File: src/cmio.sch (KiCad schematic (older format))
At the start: 28 parts, among them J1 CONN_01X02_MALE, J2 CONN_02X20, J3 USB_OTG, J4 CM3Lite, J5 CONN_COAXIAL, J6 CONN_02X20, J7 Micro_SD_Card_TFP09_2_12B, J8 CONN_01X06, SW1 SW_Push, U1 ISL91107IR, U2 LD3985M18R, U3 LD3985M28R

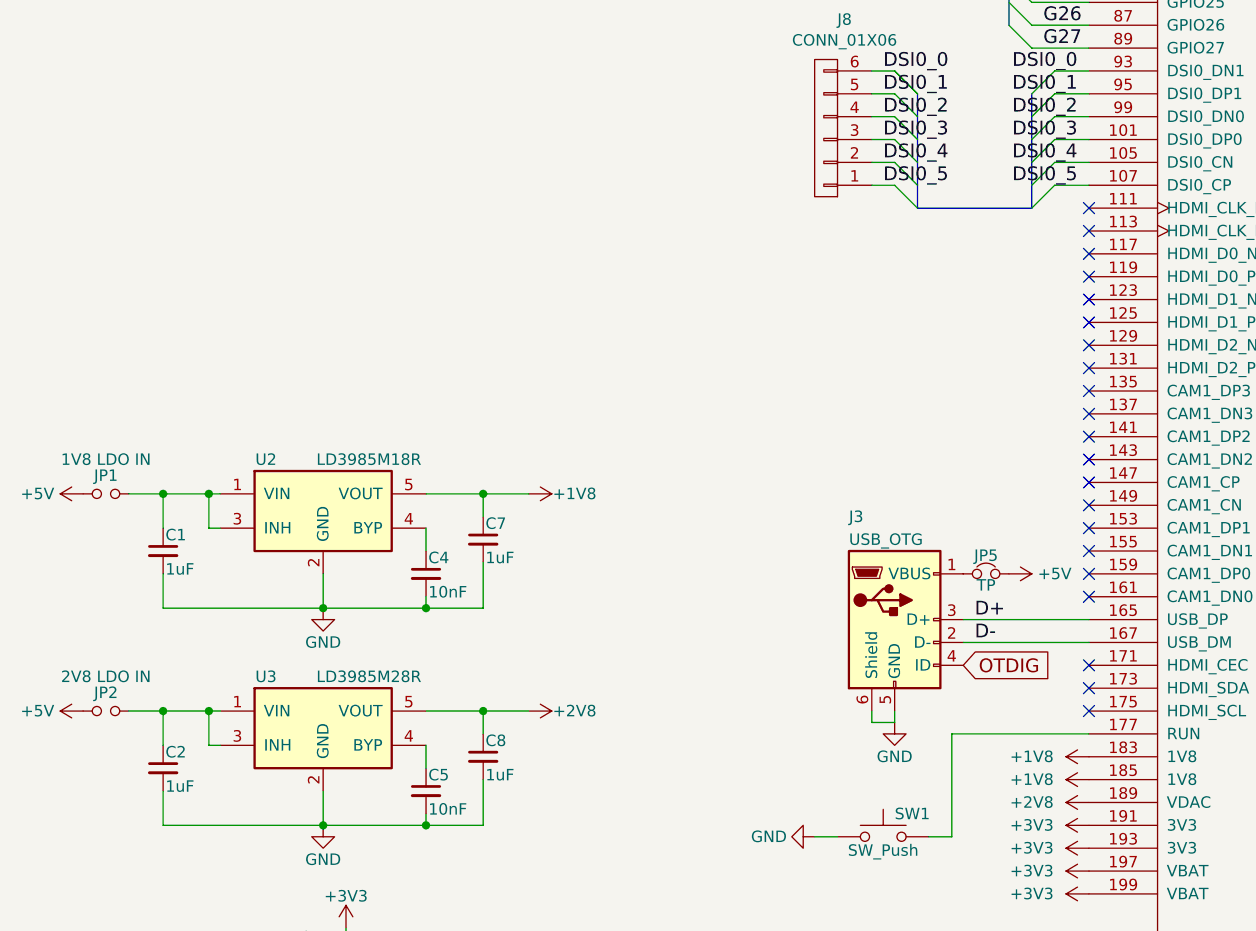
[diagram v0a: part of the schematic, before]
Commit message: Final Checks
Signed-off-by: Mahyar Koshkouei <deltabeard@users.noreply.github.com>
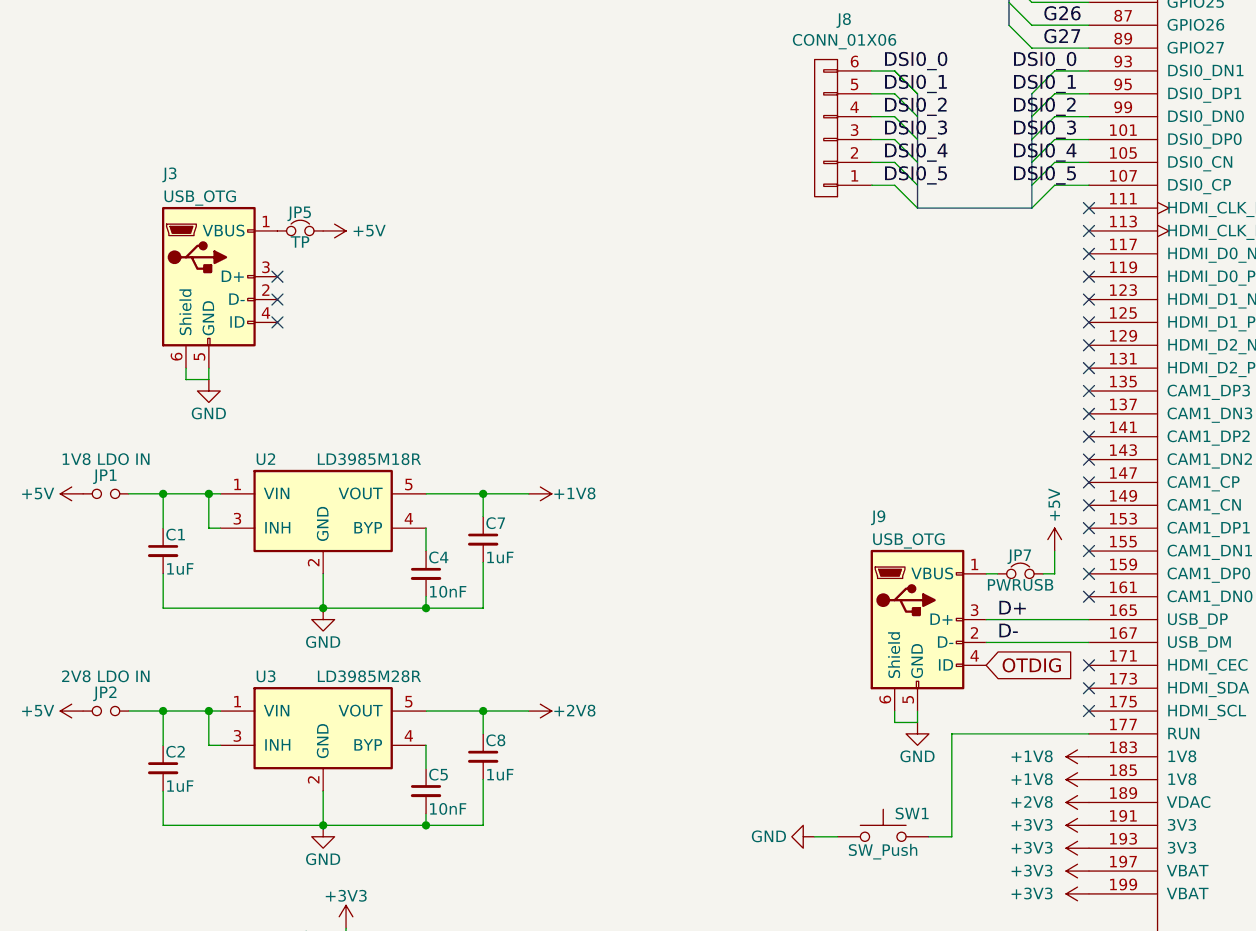
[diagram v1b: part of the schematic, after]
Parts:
- added J9: USB_OTG, foot:Micro_USB_B_10104110, symbol USB_OTG
- added JP7: PWRUSB, Pin_Headers:Pin_Header_Straight_1x02_Pitch2.54mm, symbol Jumper_NC_Small
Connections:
- net +5V: now also JP7.2
- net D+: now also J9.3 (D+); no longer J3.3 (D+)
- net D-: now also J9.2 (D-); no longer J3.2 (D-)
- net GND: now also J9.5 (GND), J9.6 (Shield)
- net OTDIG: now also J9.4 (ID); no longer J3.4 (ID)
- new net: J9.1 (VBUS), JP7.1
- no-connect marks 47 -> 50
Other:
- moved on the sheet: J3, JP5
